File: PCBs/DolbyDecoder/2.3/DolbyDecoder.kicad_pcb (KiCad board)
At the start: 2 copper layers, 95 x 55 mm, 154 parts, among them J1 Conn_01x04_Pin, J10 Conn_01x02, J11 Conn_01x04_Male, J12 Conn_01x02, J13 Conn_01x04_Male, J14 Conn_01x02_Male, J15 Conn_01x02, J16 Conn_01x02_Male, J2 Conn_01x04_Pin, J3 Conn_01x02, J4 Conn_01x02_Pin, J5 Conn_01x04_Pin, J6 Conn_01x02, J7 Conn_01x02, J8 Conn_01x02, J9 Conn_01x04_Male, U1 PCM5122PW, U2 PCM5122PW, U3 PCM5122PW, U4 SPA130, U5 AMS1117-2.5, U6 TMP100, U7 AMS1117-2.5, U8 AMS1117-3.3, X1 ECS-3225SMV-270-FP-TR

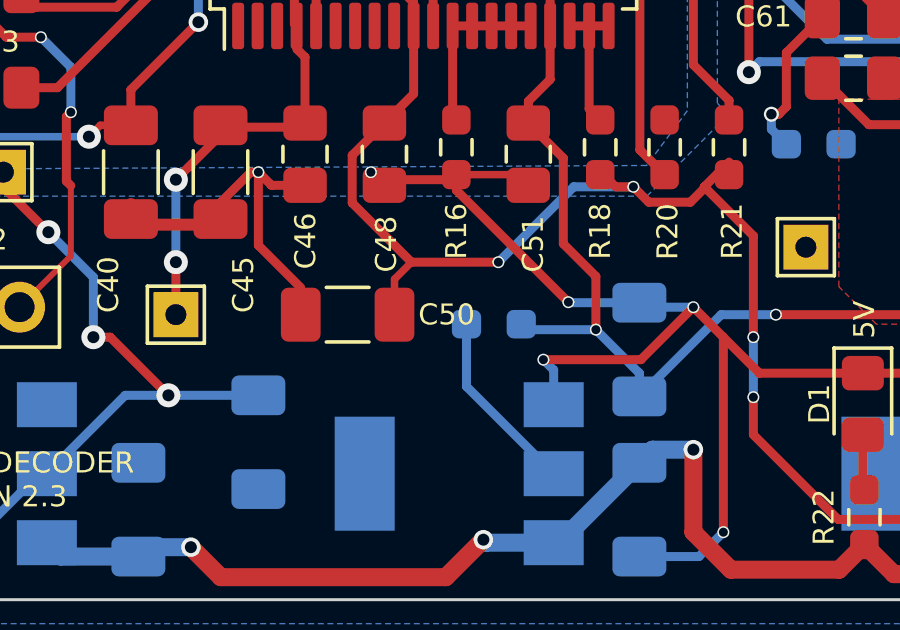
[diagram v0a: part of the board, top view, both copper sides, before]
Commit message: Mostly working
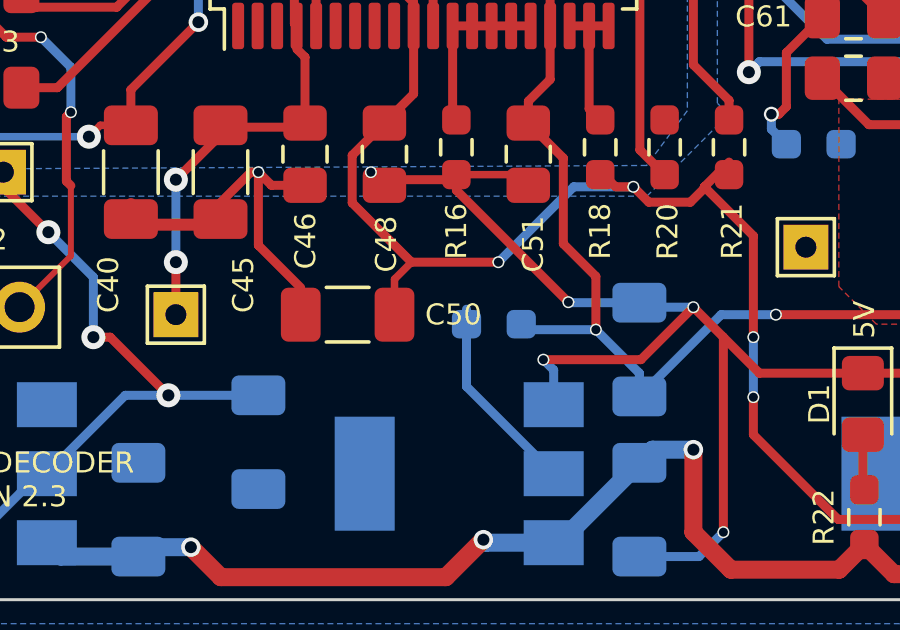
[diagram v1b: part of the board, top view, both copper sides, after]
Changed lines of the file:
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@@
     (property "ki_keywords" "capacitor cap")
     (attr smd)
-    (fp_text reference "C50" (at -3.3 0 unlocked) (layer "F.SilkS")
+    (fp_text reference "C50" (at -3.525 0 unlocked) (layer "F.SilkS")
         (effects (font (size 0.7 0.7) (thickness 0.1)))
     )
